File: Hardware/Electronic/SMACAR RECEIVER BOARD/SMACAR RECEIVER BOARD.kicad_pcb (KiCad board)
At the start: 2 copper layers, 41.5 x 70 mm, 5 parts, among them J1 M04POLAR, U1 ESP32-S3-DevKitC

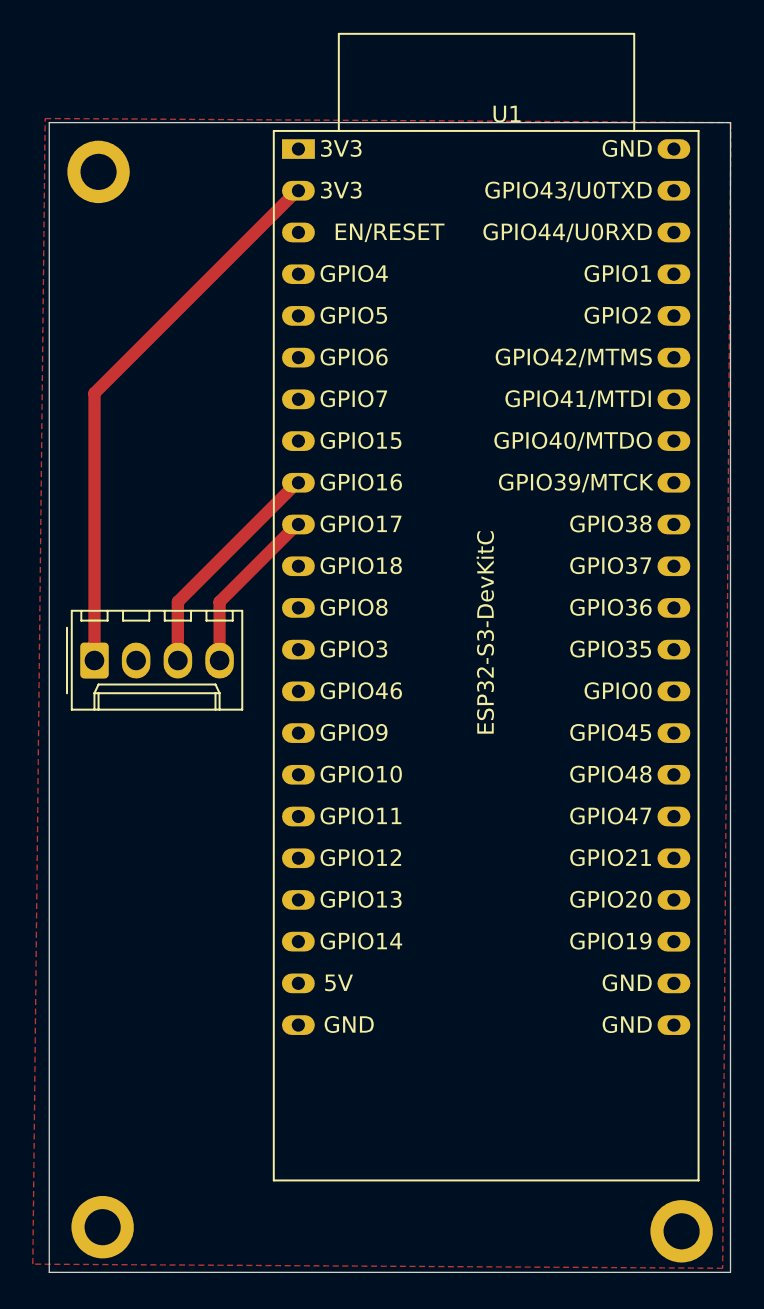
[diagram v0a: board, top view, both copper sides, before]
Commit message: PCBS
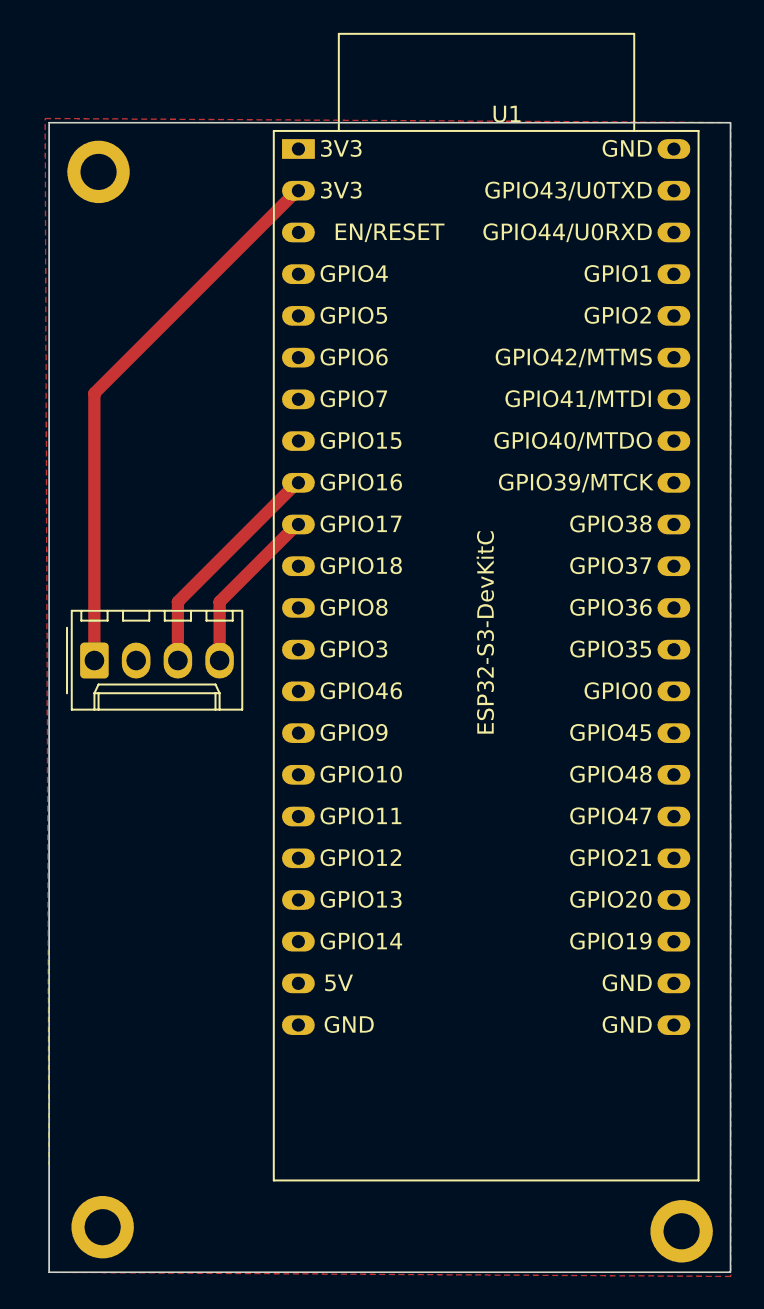
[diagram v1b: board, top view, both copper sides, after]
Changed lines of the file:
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@@
+		)
+		(fill no)
+		(layer "Edge.Cuts")
+	)
+	(gr_rect
+		(start 123.5 49.5)
+		(end 164.975 119.5)
+		(stroke
+			(width 0.05)
+			(type default)
 		)
 		(fill no)
@@
 		(hatch edge 0.5)
 		(connect_pads
-			(clearance 0.5)
+			(clearance 0.6)
 		)
-		(min_thickness 0.25)
+		(min_thickness 0.025)
 		(filled_areas_thickness no)
 		(fill yes
-			(thermal_gap 0.5)
-			(thermal_bridge_width 0.5)
+			(thermal_gap 0.6)
+			(thermal_bridge_width 0.6)
+			(island_removal_mode 1)
+			(island_area_min 10)
 		)
 		(polygon
 			(pts
-				(xy 123.25 49.25) (xy 165 49.5) (xy 164.5 119.25) (xy 122.5 119)
+				(xy 123.25 49.25) (xy 165 49.5) (xy 165 119.75) (xy 123.5 119.5)
 			)
 		)
